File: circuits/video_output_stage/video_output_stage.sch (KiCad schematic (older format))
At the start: 21 parts, among them M3 74HC04, P1 CONN_01X07, P2 CONN_01X05, P3 BNC, Q1 C5468, U1 7805

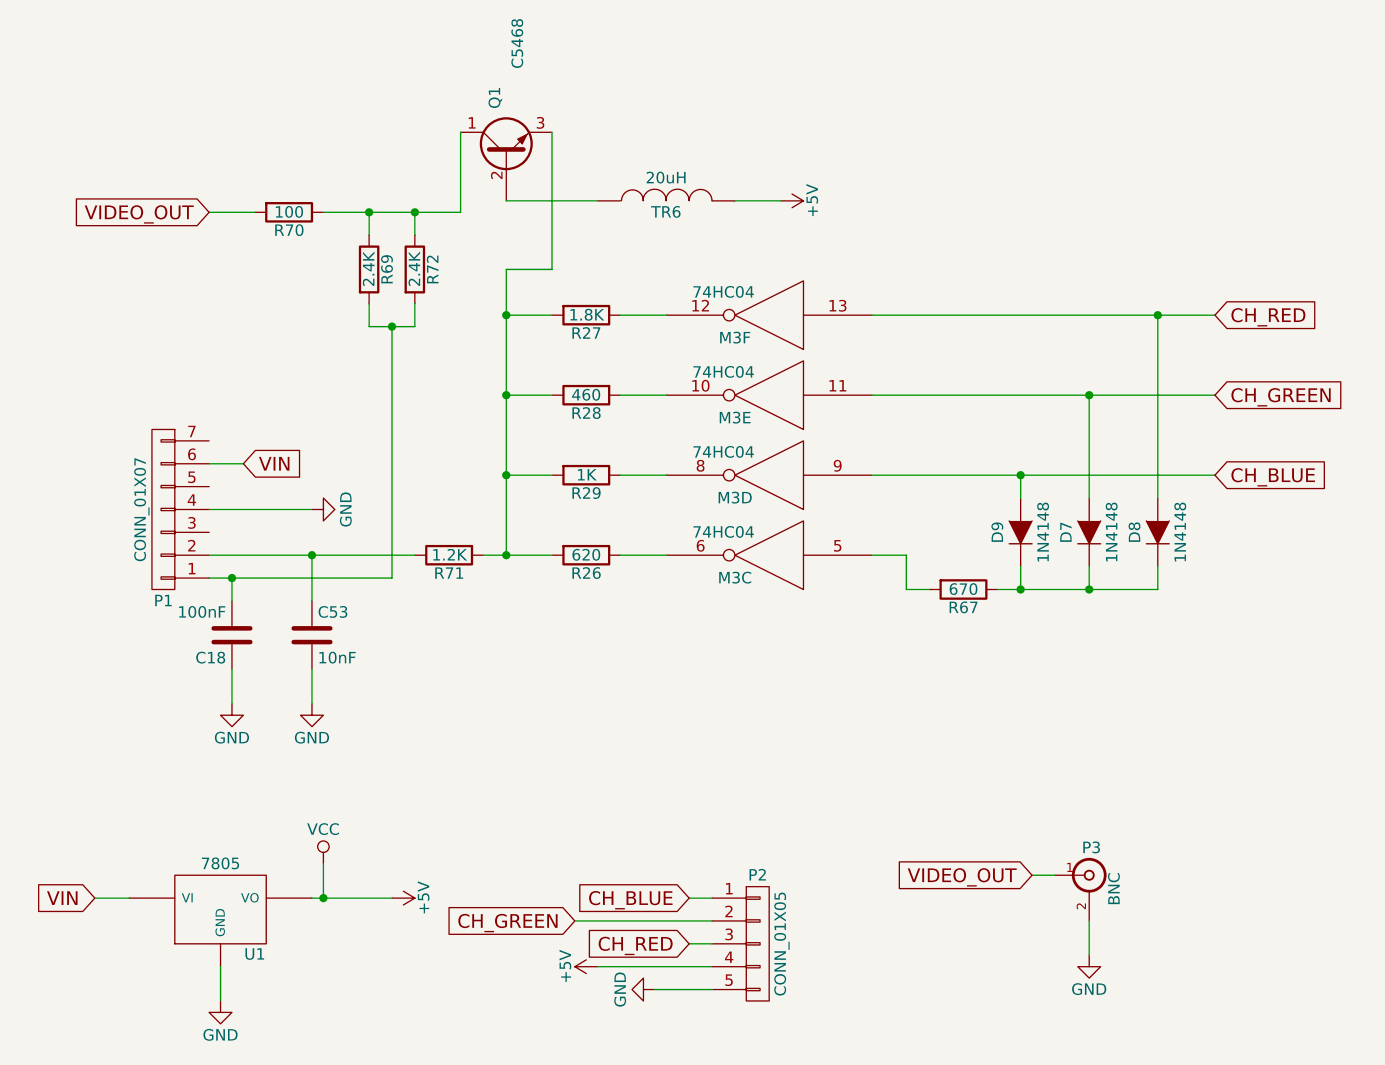
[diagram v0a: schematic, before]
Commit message: circuit's pretty much done; now for a new board
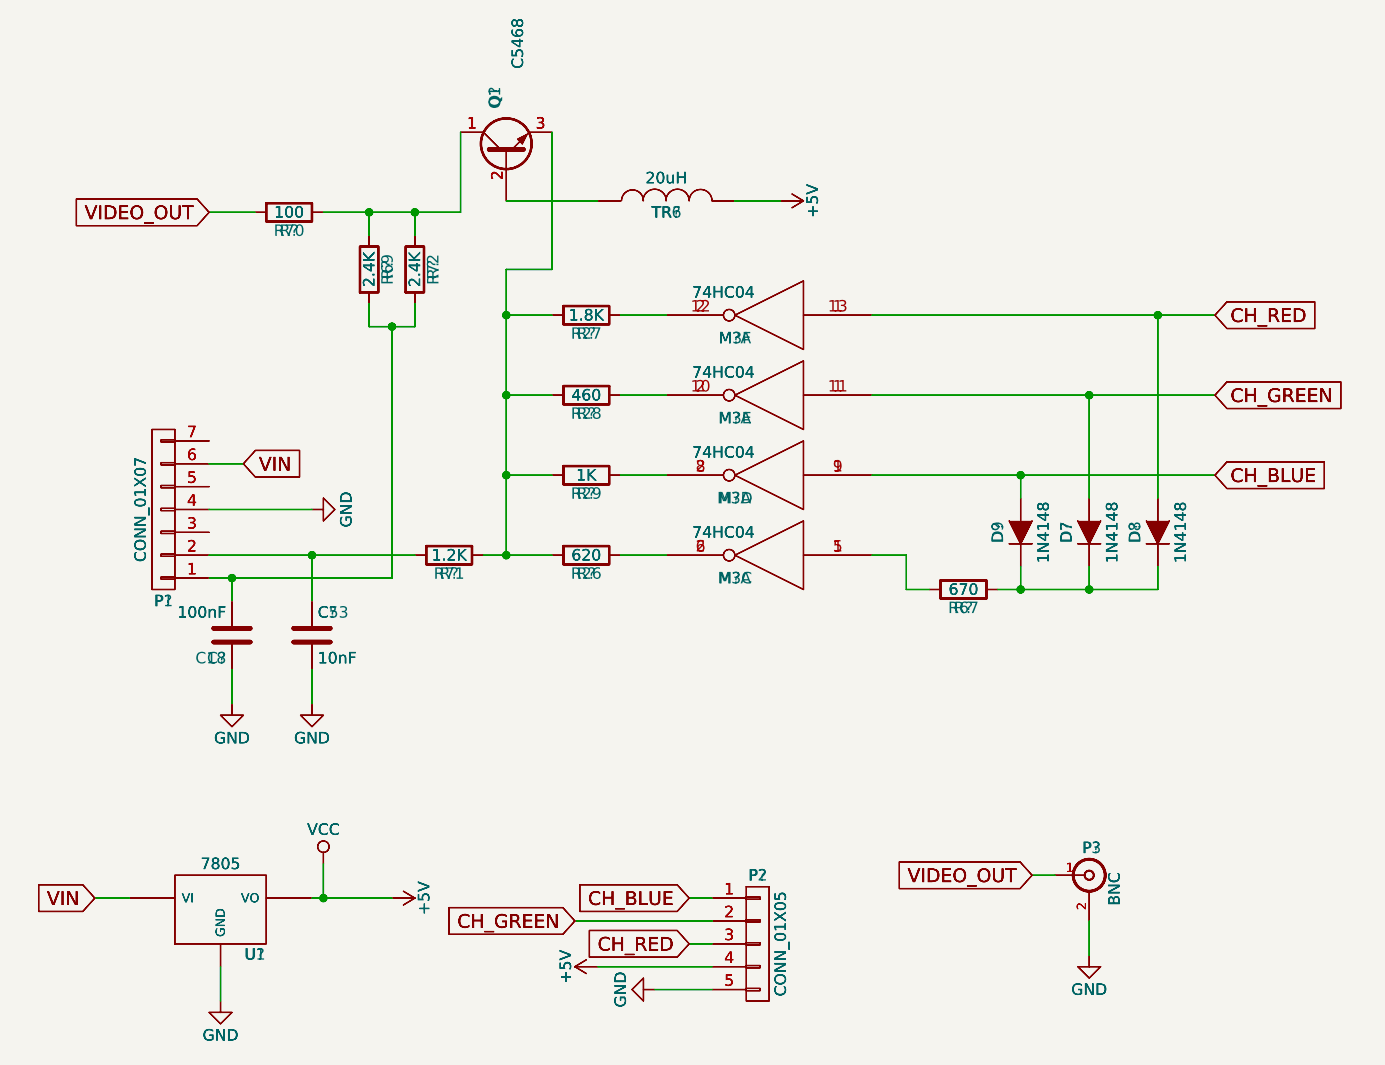
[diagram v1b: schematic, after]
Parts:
- added C?: 100nF, Capacitors_ThroughHole:C_Disc_D6_P5, symbol C
- added C?: 10nF, Capacitors_ThroughHole:C_Disc_D6_P5, symbol C
- added D? (x3): 1N4148, Diodes_ThroughHole:Diode_DO-35_SOD27_Horizontal_RM10, symbol D
- added M? (x4): 74HC04, Housings_DIP:DIP-14_W7.62mm_LongPads, symbol 74HC04
- added P?: CONN_01X07, Connectors_Phoenix:PhoenixContact_MSTBVA-G_07x5.00mm_Vertical, symbol CONN_01X07
- added P?: CONN_01X05, Pin_Headers:Pin_Header_Straight_1x05, symbol CONN_01X05
- added P?: BNC, Connect:PINHEAD1-2, symbol BNC
- added Q?: C5468, TO_SOT_Packages_THT:TO-92_Inline_Wide, symbol Q_NPN_CBE
- added R?: 100, Resistors_ThroughHole:Resistor_Horizontal_RM15mm, symbol R
- added R? (x2): 2.4K, Resistors_ThroughHole:Resistor_Horizontal_RM15mm, symbol R
- added R?: 1.2K, Resistors_ThroughHole:Resistor_Horizontal_RM15mm, symbol R
- added R?: 1.8K, Resistors_ThroughHole:Resistor_Horizontal_RM15mm, symbol R
- added R?: 460, Resistors_ThroughHole:Resistor_Horizontal_RM15mm, symbol R
- added R?: 1K, Resistors_ThroughHole:Resistor_Horizontal_RM15mm, symbol R
- added R?: 620, Resistors_ThroughHole:Resistor_Horizontal_RM15mm, symbol R
- added R?: 670, Resistors_ThroughHole:Resistor_Horizontal_RM15mm, symbol R
- added TR?: 20uH, Choke_Axial_ThroughHole:Choke_Horizontal_RM20mm, symbol INDUCTOR
- added U?: 7805, TO_SOT_Packages_THT:TO-220_Neutral123_Vertical_LargePads, symbol 7805
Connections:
- net +5V: now also M?.14 (VCC), M?.14 (VCC), M?.14 (VCC), M?.14 (VCC), P?.4 (P4), TR?.2, U?.3 (VO)
- net CH_BLUE: now also D?.2 (A), M?.1, P?.1 (P1)
- net CH_GREEN: now also D?.2 (A), M?.1, P?.2 (P2)
- net CH_RED: now also D?.2 (A), M?.1, P?.3 (P3)
- net GND: now also C?.1, C?.2, M?.7 (GND), M?.7 (GND), M?.7 (GND), M?.7 (GND), P?.2 (Ext), P?.4 (P4), P?.5 (P5), U?.2 (GND)
- net VIDEO_OUT: now also P?.1 (In), R?.2
- net VIN: now also P?.6 (P6), U?.1 (VI)
- net at C18.2, P1.1 (P1), R69.2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: now also C?.2, P?.1 (P1), R?.2, R?.2
- net at C53.1, P1.2 (P2), R71.1: now also C?.1, P?.2 (P2), R?.1
- net at P1.3 (P3): now also P?.3 (P3)
- net at P1.5 (P5): now also P?.5 (P5)
- net at P1.7 (P7): now also P?.7 (P7)
- net at Q1.1 (C), R69.1, R70.1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: now also Q?.1 (C), R?.1, R?.1, R?.1
- net at Q1.3 (E), R26.2, R27.2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: now also Q?.3 (E), R?.1, R?.2, R?.2, R?.2, R?.2
- net at M3.12, R27.1: now also M?.2, R?.1
- net at M3.10, R28.2: now also M?.2, R?.2
- net at M3.8, R29.1: now also M?.2, R?.1
- net at M3.6, R26.1: now also M?.2, R?.1
- net at M3.5, R67.2: now also M?.1, R?.2
- net at D7.1 (K), D8.1 (K), D9.1 (K)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: now also D?.1 (K), D?.1 (K), D?.1 (K), R?.1
- net at Q1.2 (B), TR6.1: now also Q?.2 (B), TR?.1
